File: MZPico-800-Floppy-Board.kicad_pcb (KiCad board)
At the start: 2 copper layers, 115.3 x 92.9 mm, 9 parts, among them J1 MZ800_Expansion_Bus, J2 SHUGART, J3 PC Floppy, U1 SN74LVC245APW, U2 SN74LVC245APW

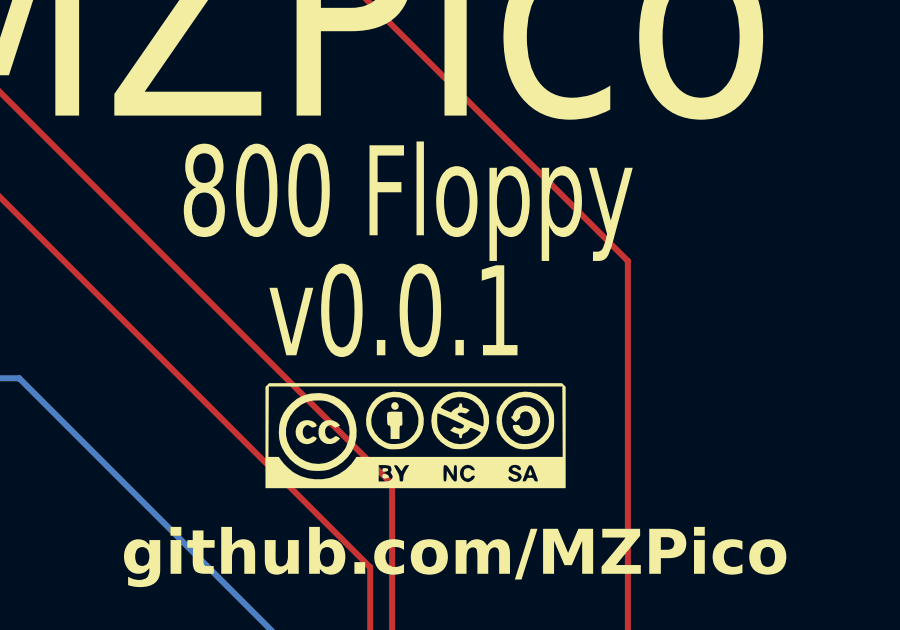
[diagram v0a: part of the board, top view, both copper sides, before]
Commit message: Reset board version
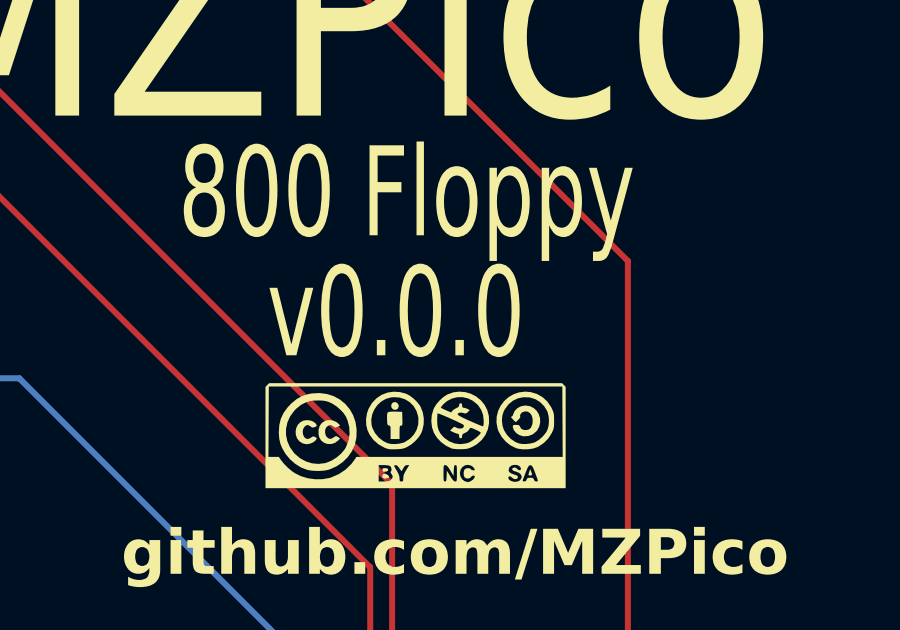
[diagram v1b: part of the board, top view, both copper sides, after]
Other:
- board text added: "v0.0.0"
- board text removed: "v0.0.1"
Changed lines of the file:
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@@
 		)
 	)
-	(gr_text "v0.0.1"
+	(gr_text "v0.0.0"
 		(at 181.26 86.8 0)
 		(layer "F.SilkS")

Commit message: chore: update version on PCB to v0.0.1
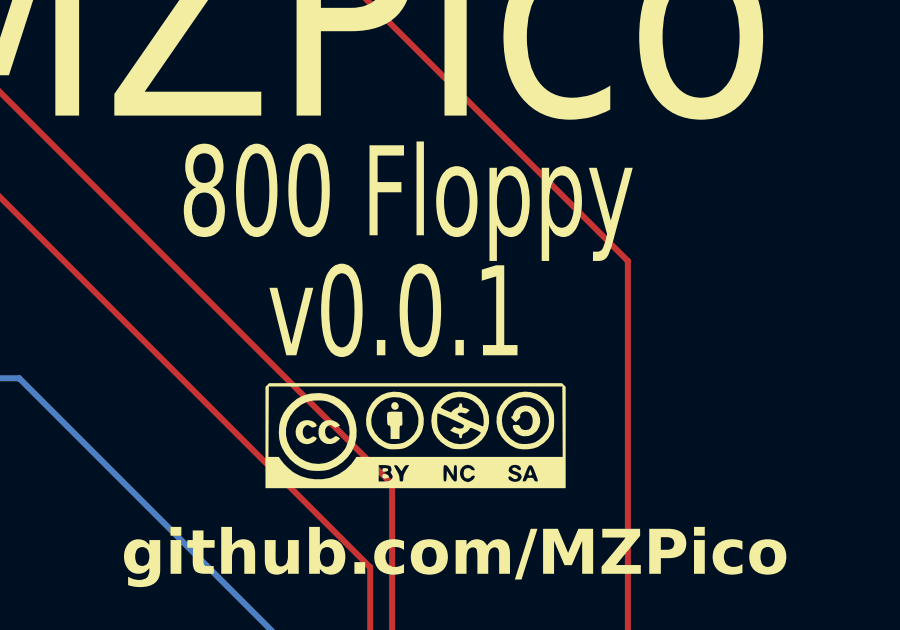
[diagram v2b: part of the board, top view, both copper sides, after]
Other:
- board text added: "v0.0.1"
- board text removed: "v0.0.0"
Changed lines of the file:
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@@
 		)
 	)
-	(gr_text "v0.0.0"
+	(gr_text "v0.0.1"
 		(at 181.26 86.8 0)
 		(layer "F.SilkS")
